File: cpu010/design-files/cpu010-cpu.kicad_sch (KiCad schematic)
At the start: 16 parts, among them SW201 Reset, U201 MC68010P, U202 74ACT05, U203 DS1813, Y201 40MHz

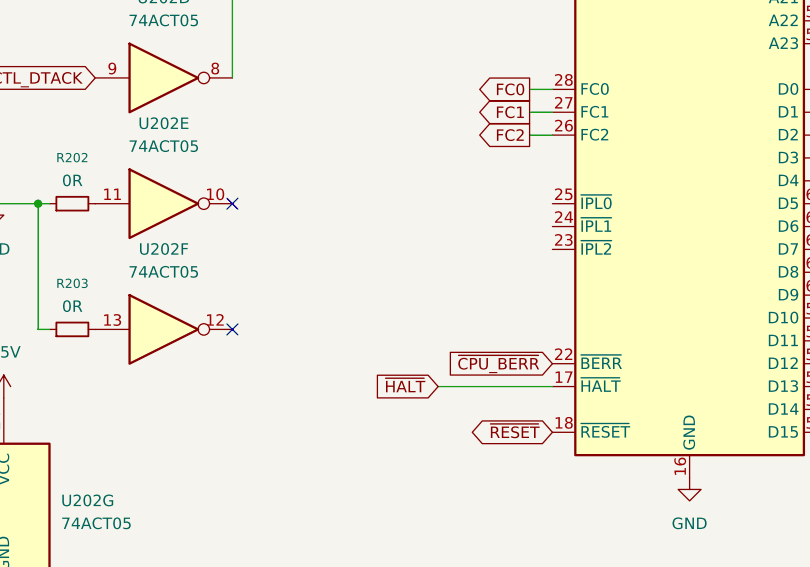
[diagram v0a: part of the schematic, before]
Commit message: Route a bunch of I/O controller signals.
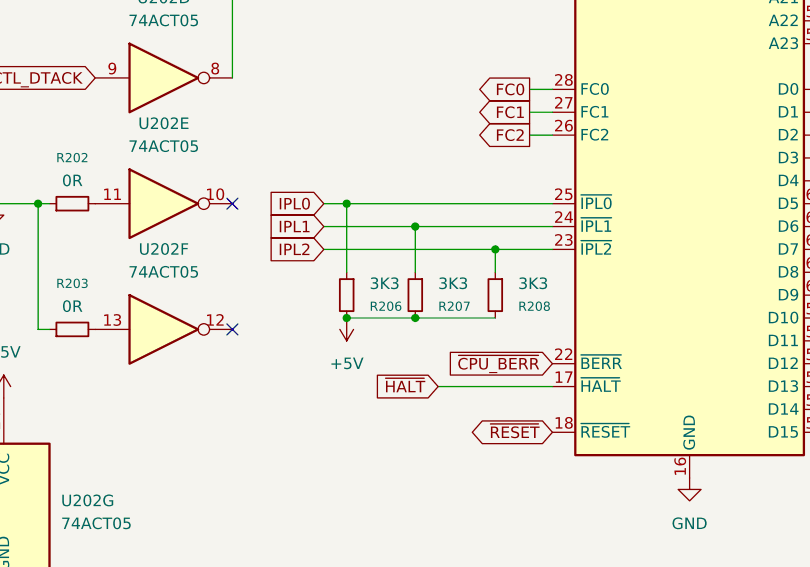
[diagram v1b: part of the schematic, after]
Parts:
- added R206, R207, R208: 3K3, Resistor_SMD:R_0805_2012Metric_Pad1.20x1.40mm_HandSolder, symbol Device:R_Small
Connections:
- net +5V: now also R206.2, R207.2, R208.2
- net IPL2: now reaches U201.23 (~{IPL2})
- net IPL2: now also R208.1
- net IPL1: now reaches U201.24 (~{IPL1})
- net IPL1: now also R207.1
- net IPL0: now reaches U201.25 (~{IPL0})
- net IPL0: now also R206.1
